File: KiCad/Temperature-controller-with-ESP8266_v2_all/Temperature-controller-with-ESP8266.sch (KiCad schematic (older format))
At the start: 59 parts, among them J1 USB_B_Micro, J10 Conn_01x08_Male, J2 Conn_01x04_Male, J3 Conn_01x04_Female, J4 Conn_01x03_Male, J5 RJ13, J6 Conn_01x03_Male, J7 Screw_Terminal_01x02, J8 Screw_Terminal_01x02, J9 Conn_01x08_Male, Q1 SS8050-H, Q2 SS8050-H, Q3 MMBT5551L, Q4 MMBT5551L, SW1 SW_Push, SW2 SW_Push_SPDT, U1 ESP-12F, U2 CH340G, U3 EL817, U4 EL817, U5 AMS1117-3.3, U6 M24512-EEPROM, Y1 Crystal_GND24

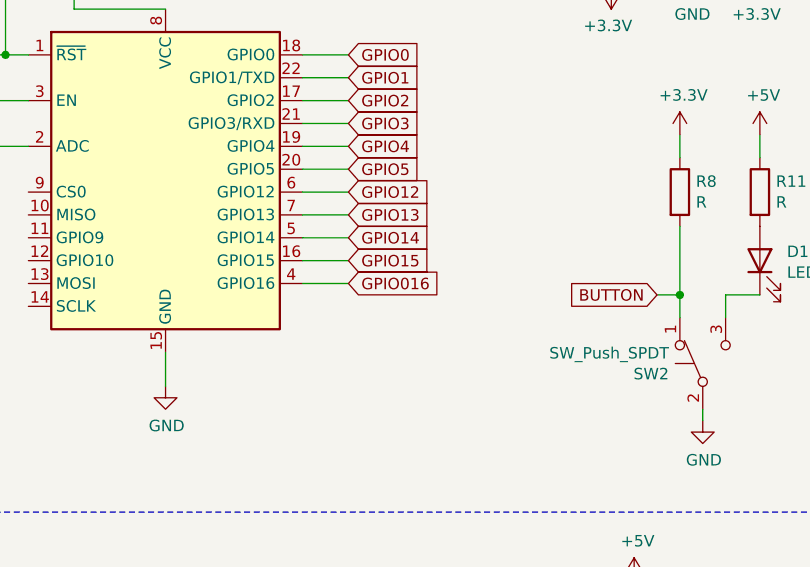
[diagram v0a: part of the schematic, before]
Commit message: Test of Git+ module atom
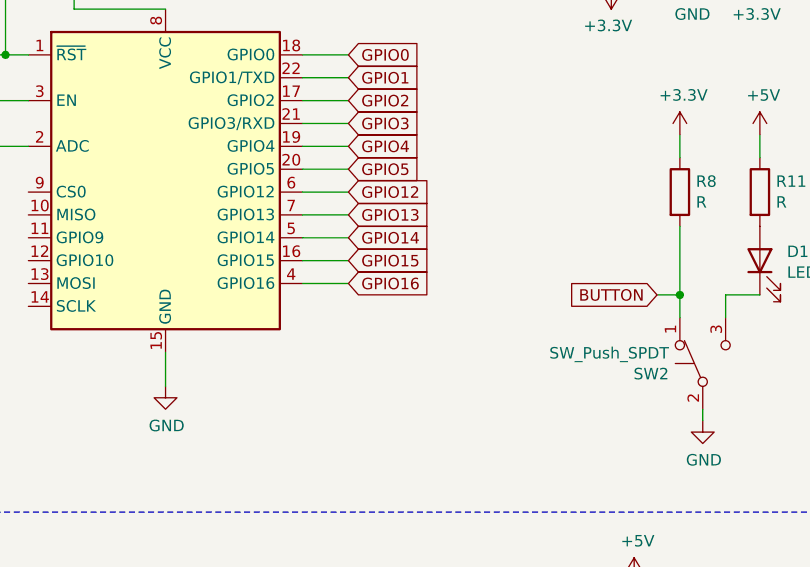
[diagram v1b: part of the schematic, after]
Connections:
- net GPIO016 is gone; now on net BUTTON: U1.4 (GPIO16)
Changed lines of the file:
@@
 BUTTON
 Text GLabel 3350 3000 2    50   Input ~ 0
-GPIO016
+GPIO16
 Wire Wire Line
 	3350 3000 3150 3000
